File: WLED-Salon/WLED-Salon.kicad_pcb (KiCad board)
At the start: 2 copper layers, 2 parts, among them U1 ESP32-DevKitC, U2 74AHCT125

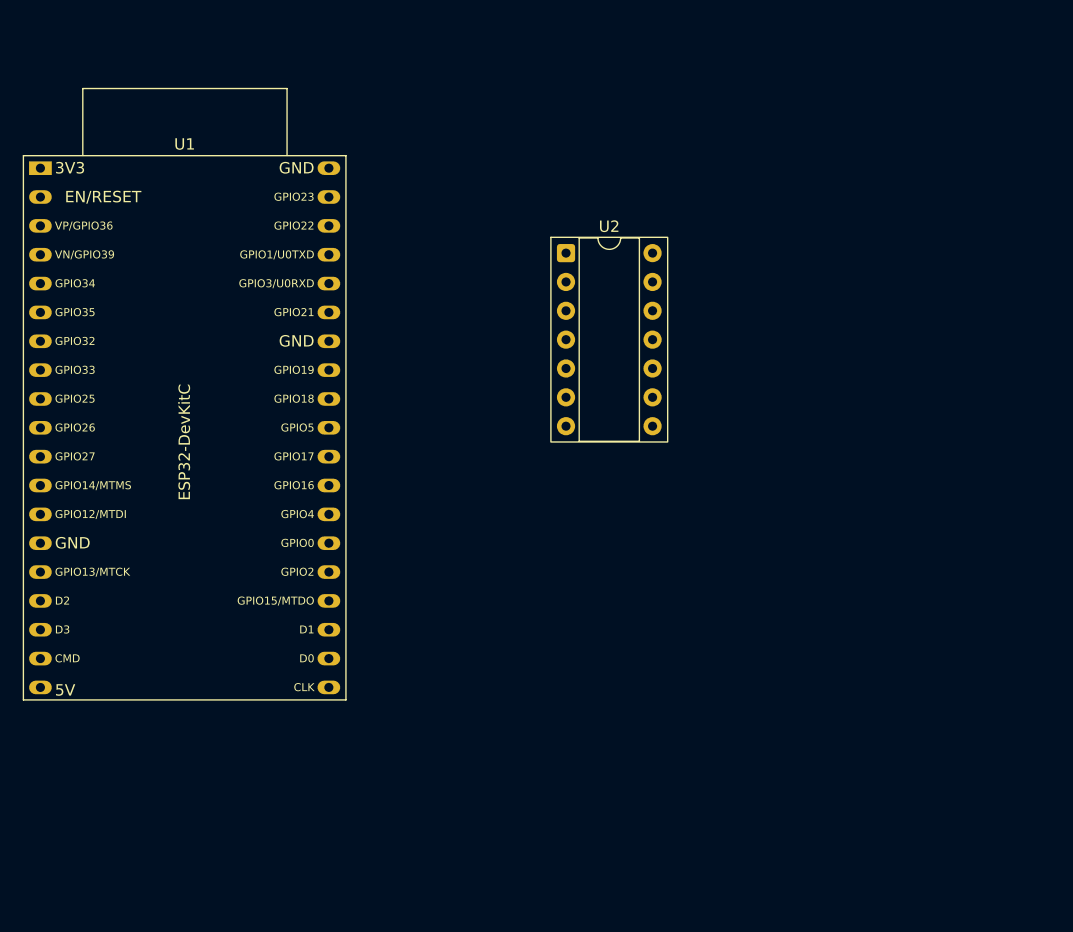
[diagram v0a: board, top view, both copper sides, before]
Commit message: pcs done mostly
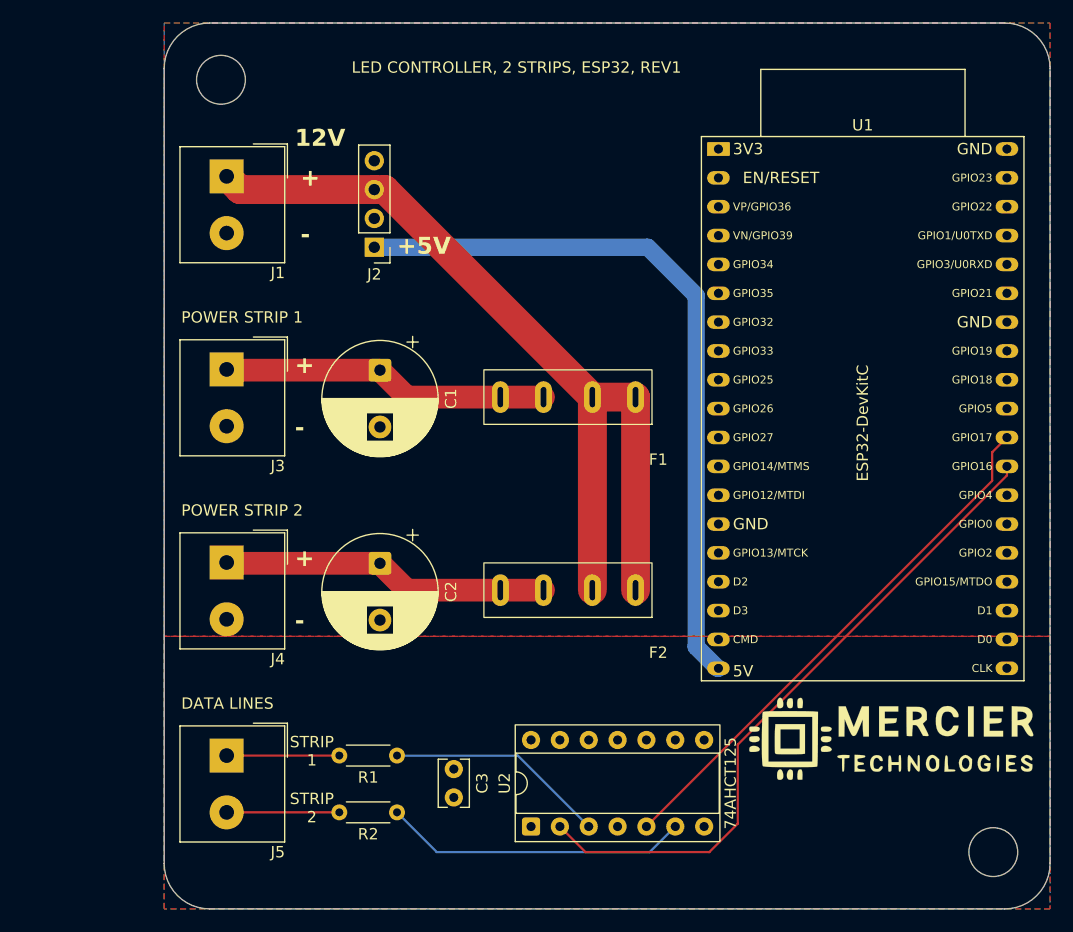
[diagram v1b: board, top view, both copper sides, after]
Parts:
- added C1: 1000uF 16V, Capacitor_THT:CP_Radial_D10.0mm_P5.00mm, F.Cu at (144.0, 77.6)
- added C2: 1000uF 16V, Capacitor_THT:CP_Radial_D10.0mm_P5.00mm, F.Cu at (144.0, 94.6)
- added C3: 100nF, Capacitor_THT:C_Rect_L4.0mm_W2.5mm_P2.50mm, F.Cu at (150.5, 112.7)
- added F1: Fuse 5A, fuse-lib:micro fuse holder, F.Cu at (166.5, 79.9)
- added F2: Fuse 5A, fuse-lib:micro fuse holder, F.Cu at (166.5, 96.9)
- added G***: LOGO, LOGO:merciertech600, F.Cu at (189.0, 110.0)
- added J1: 12V Power Supply, TerminalBlock_Altech:Altech_AK100_1x02_P5.00mm, F.Cu at (130.5, 60.5)
- added J2: Buck Converter, Connector_PinHeader_2.54mm:PinHeader_1x04_P2.54mm_Vertical, F.Cu at (143.5, 66.7)
- added J3: Power LED Strip 1, TerminalBlock_Altech:Altech_AK100_1x02_P5.00mm, F.Cu at (130.5, 77.5)
- added J4: Power LED Strip 2, TerminalBlock_Altech:Altech_AK100_1x02_P5.00mm, F.Cu at (130.5, 94.5)
- added J5: LED Strip Data 1 & 2, TerminalBlock_Altech:Altech_AK100_1x02_P5.00mm, F.Cu at (130.5, 111.5)
- added R1: 62 Ohm, Resistor_THT:R_Axial_DIN0204_L3.6mm_D1.6mm_P5.08mm_Horizontal, F.Cu at (145.5, 111.5)
- added R2: 62 Ohm, Resistor_THT:R_Axial_DIN0204_L3.6mm_D1.6mm_P5.08mm_Horizontal, F.Cu at (145.5, 116.5)
- added REF**: MountingHole_4.3mm_M4, MountingHole:MountingHole_4.3mm_M4, F.Cu at (198.0, 120.0)
- added REF**: MountingHole_4.3mm_M4, MountingHole:MountingHole_4.3mm_M4, F.Cu at (130.0, 52.0)
- moved U1 59.7 mm to (173.8, 58.1)
- moved U2 50.6 mm to (157.3, 117.7), turned to 90 degrees
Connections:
- U1 pad 14: Net-(U1-GND-Pad14) -> GND
- U1 pad 19: unconnected-(U1-5V-Pad19) -> +5V
- U1 pad 27: unconnected-(U1-GPIO16-Pad27) -> GPIO16
- U1 pad 28: unconnected-(U1-GPIO17-Pad28) -> GPIO17
- U1 pad 32: Net-(U1-GND-Pad14) -> GND
- U1 pad 38: Net-(U1-GND-Pad14) -> GND
- U2 pad 1: unconnected-(U2-Pad1) -> GND
- U2 pad 10: (no net) -> +5V
- U2 pad 11: (no net) -> unconnected-(U2-Pad11)
- U2 pad 12: (no net) -> GND
- U2 pad 13: (no net) -> +5V
- U2 pad 14: unconnected-(U2E-VCC-Pad14) -> +5V
- U2 pad 2: unconnected-(U2-Pad2) -> GPIO16
- U2 pad 3: unconnected-(U2-Pad3) -> Net-(R1-Pad1)
- U2 pad 4: unconnected-(U2-Pad4) -> GND
- U2 pad 5: unconnected-(U2-Pad5) -> GPIO17
- U2 pad 6: unconnected-(U2-Pad6) -> Net-(R2-Pad1)
- U2 pad 7: unconnected-(U2E-GND-Pad7) -> GND
- U2 pad 8: (no net) -> unconnected-(U2-Pad8)
- U2 pad 9: (no net) -> GND
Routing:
- net +12V: track 0.00 -> 78.1 mm
- net +5V: track 0.00 -> 63.8 mm
- net GPIO16: track 0.00 -> 58.9 mm
- net GPIO17: track 0.00 -> 47.4 mm
- net Net-(J4-Pin_1): track 0.00 -> 28.9 mm
- net Net-(J3-Pin_1): track 0.00 -> 28.9 mm
- net Net-(R2-Pad1): track 0.00 -> 26.9 mm
- net Net-(R1-Pad1): track 0.00 -> 19.5 mm
- net DATA2: track 0.00 -> 9.92 mm
- net DATA1: track 0.00 -> 9.92 mm
- added copper zone on F.Cu, net +12V
- added copper zone on F.Cu, net +5V
- added copper zone on B.Cu, net GND
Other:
- board outline added: 78 x 78 mm
- board text added: "+"
- board text added: "+5V"
- board text added: "-"
- board text added: "12V"
- board text added: "DATA LINES"
- board text added: "LED CONTROLLER, 2 STRIPS, ESP32, REV1"
- board text added: "POWER STRIP 1"
- board text added: "POWER STRIP 2"
- board text added: "STRIP 1"
- board text added: "STRIP 2"
